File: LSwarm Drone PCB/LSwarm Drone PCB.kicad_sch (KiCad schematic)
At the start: 128 parts, among them J1 Conn_01x04_Pin, J3 JST / BT2.0 Connector, J4 Conn_01x02_Pin, J5 Conn_01x02_Pin, J6 Conn_01x02_Pin, J7 Conn_01x02_Pin, Q1 AO3400A, Q2 AO3400A, Q3 AO3400A, Q4 AO3400A, Q7 AO3407A, SW1 MSK12C02, SW2 SKRPACE010, SW3 SKRPACE010, SW4 SKRPACE010, SW5 SKRPACE010, U1 LSM6DSRTR, U12 AP2112K-3.3, U3 TPS61023DRLR, U4 SN74LVC1T45DBVR, U5 BMP581, X1 X322512MSB4SI

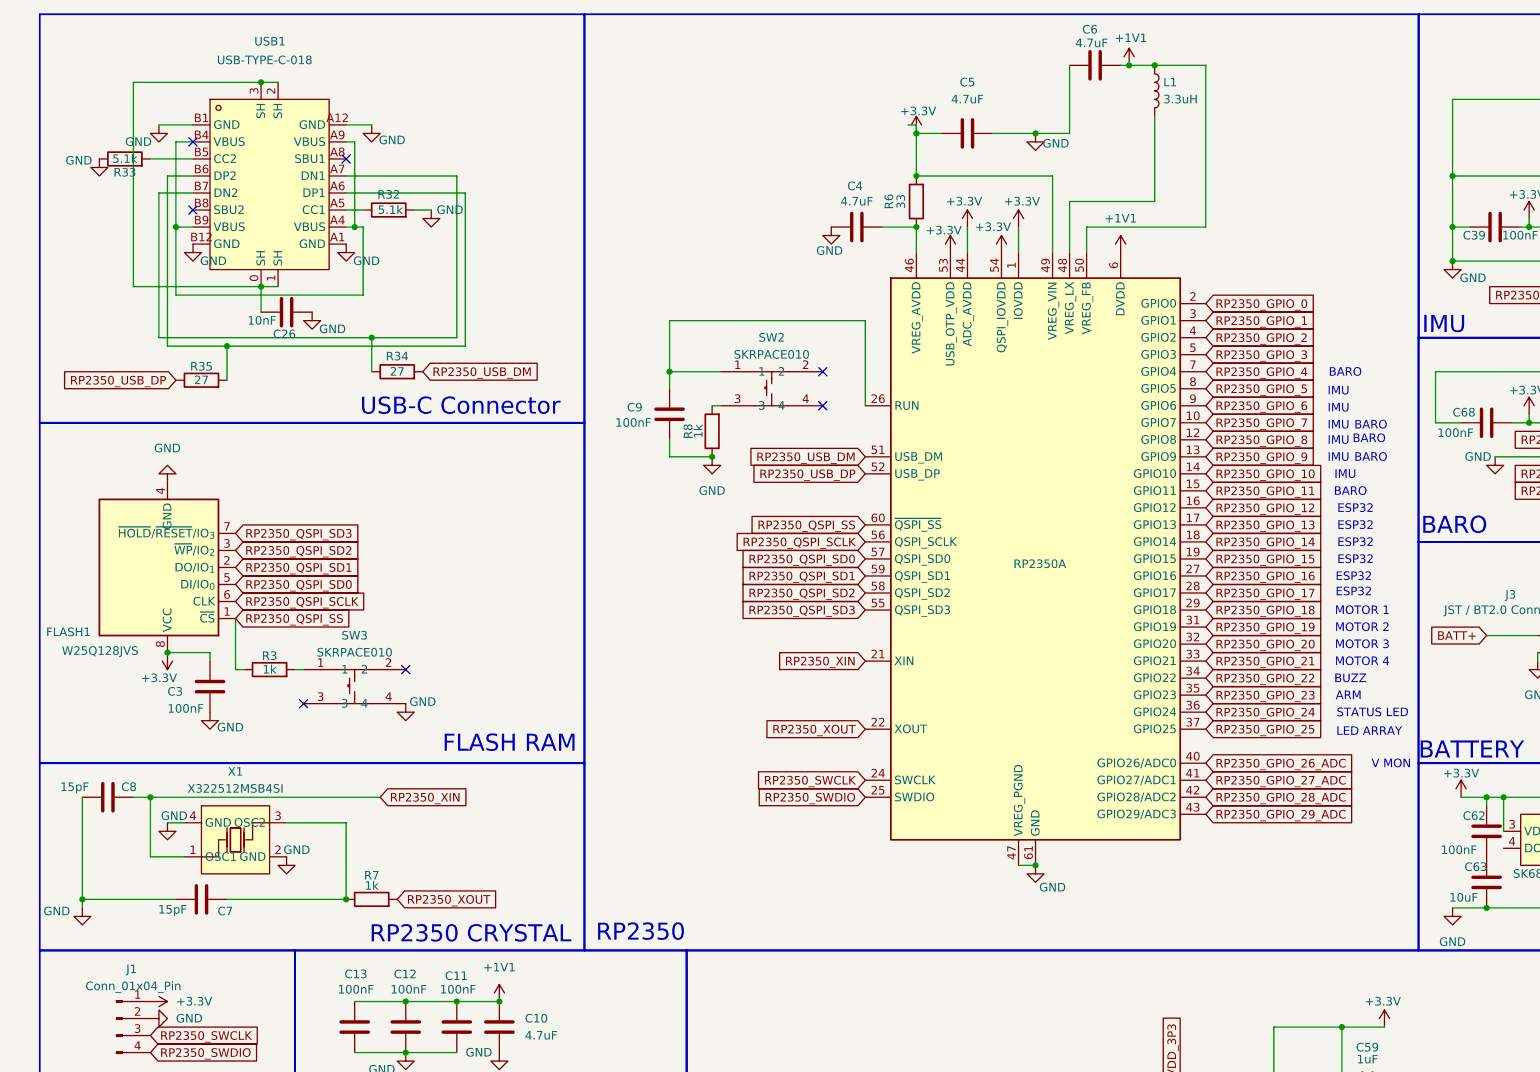
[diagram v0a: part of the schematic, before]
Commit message: sync
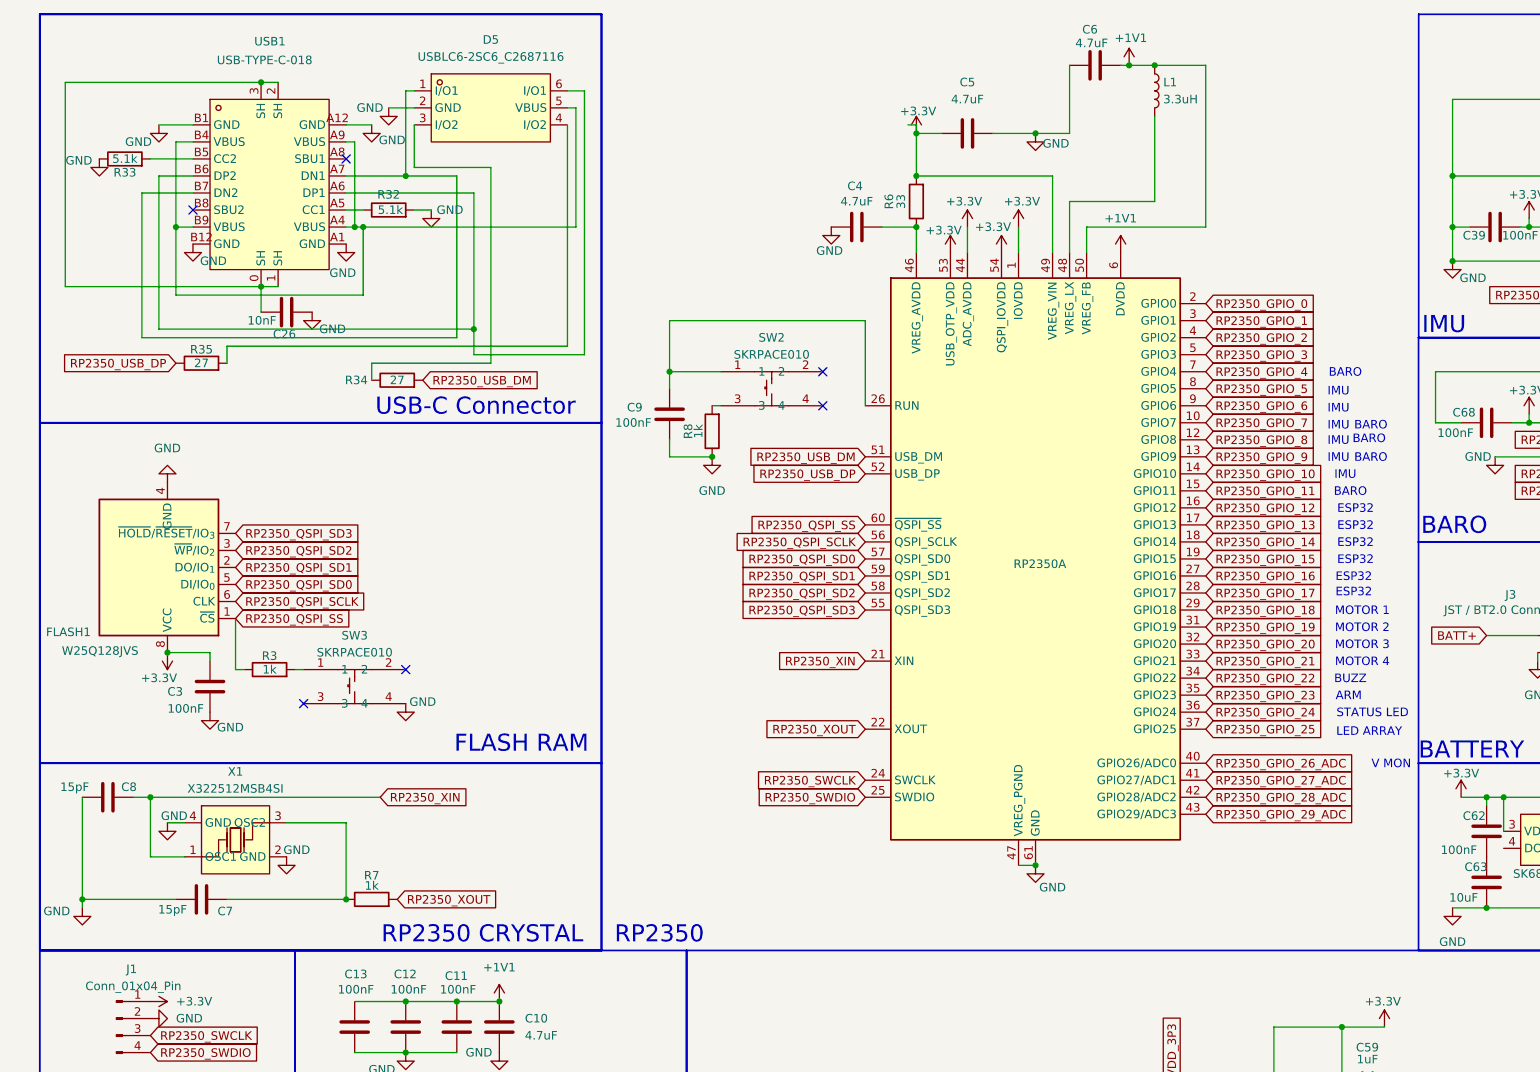
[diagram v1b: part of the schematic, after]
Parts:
- added D5: USBLC6-2SC6_C2687116, easyeda2kicad:SOT-23-6_L2.9-W1.6-P0.95-LS2.8-BL, symbol easyeda2kicad:USBLC6-2SC6_C2687116
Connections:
- net GND: now also D5.2 (GND)
- net at USB1.A6 (DP1), USB1.B6 (DP2): now also D5.6 (I/O1); no longer R35.2
- net at USB1.A7 (DN1), USB1.B7 (DN2): now also D5.1 (I/O1); no longer R34.1
- net at USB1.A4 (VBUS), USB1.A9 (VBUS), USB1.B4 (VBUS)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: now also D5.5 (VBUS)
- new net: D5.3 (I/O2), R34.1
- new net: D5.4 (I/O2), R35.2
- no-connect marks 31 -> 30
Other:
- moved on the sheet: R34, R35
